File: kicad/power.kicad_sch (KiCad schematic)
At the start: 79 parts, among them J3 Conn_01x01_Pin, J9 Conn_01x02_Pin, U11 AMS1117-5.0, U12 ACS711xEXLT-15AB, U13 LM2937xMP, U15 MAX40200AUK, U7 AMS1117-3.3, U8 ACS711xEXLT-15AB, U9 ACS711xEXLT-15AB

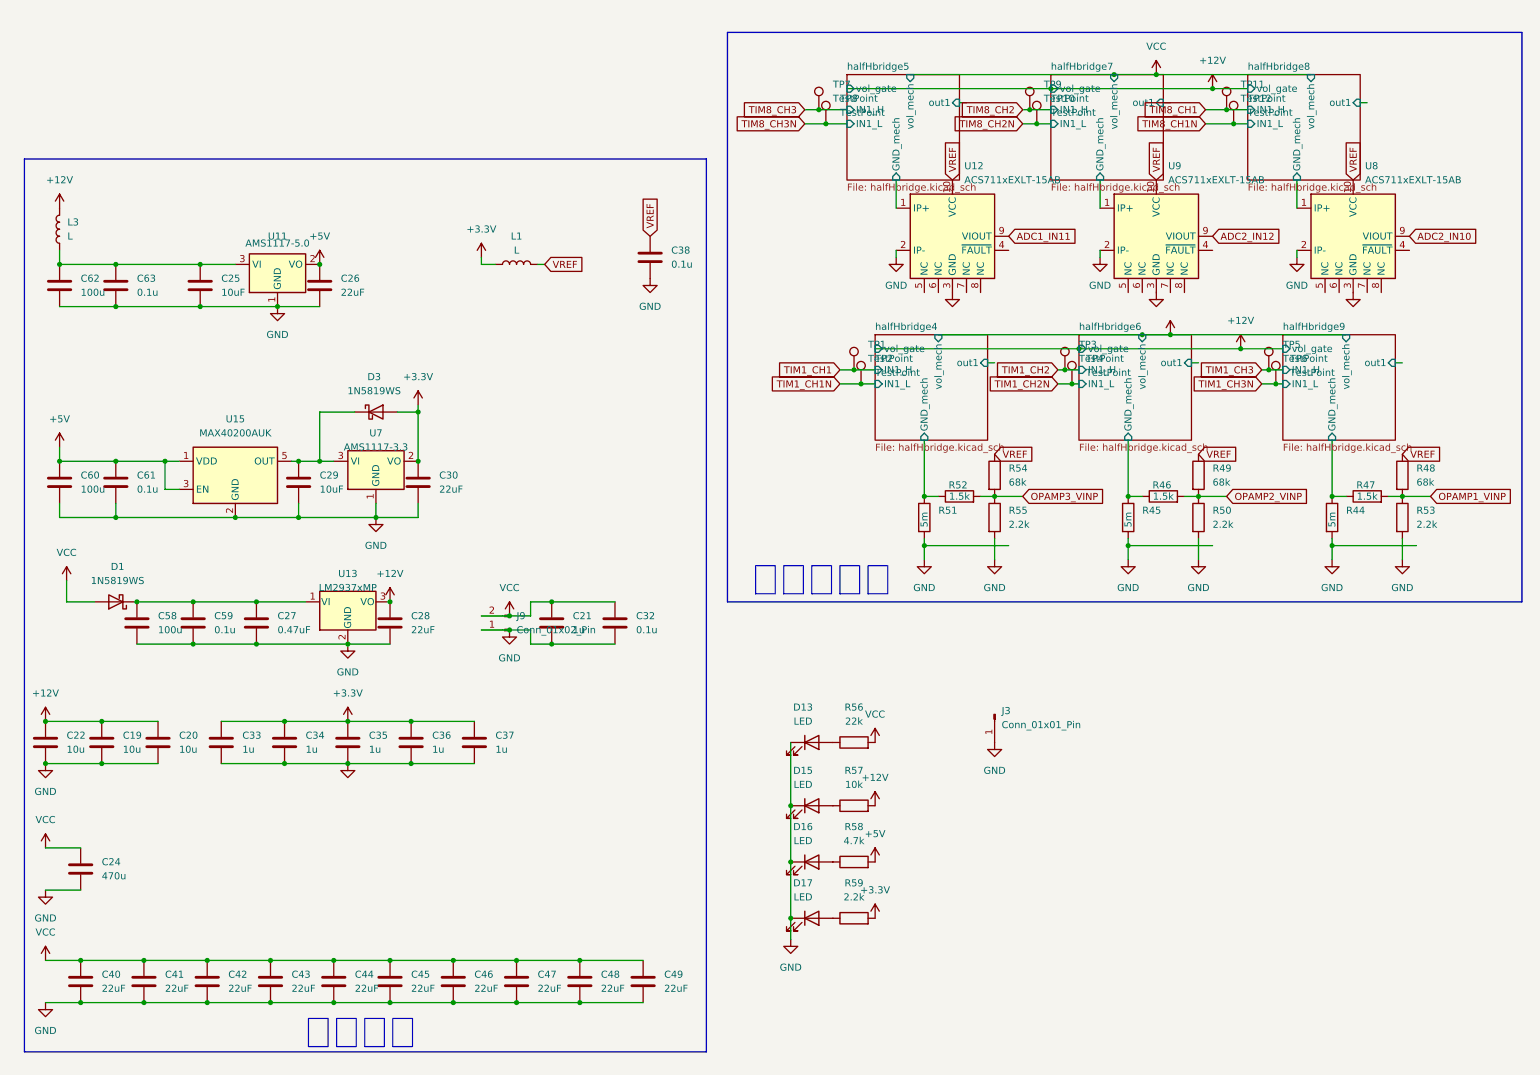
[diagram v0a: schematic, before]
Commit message: a
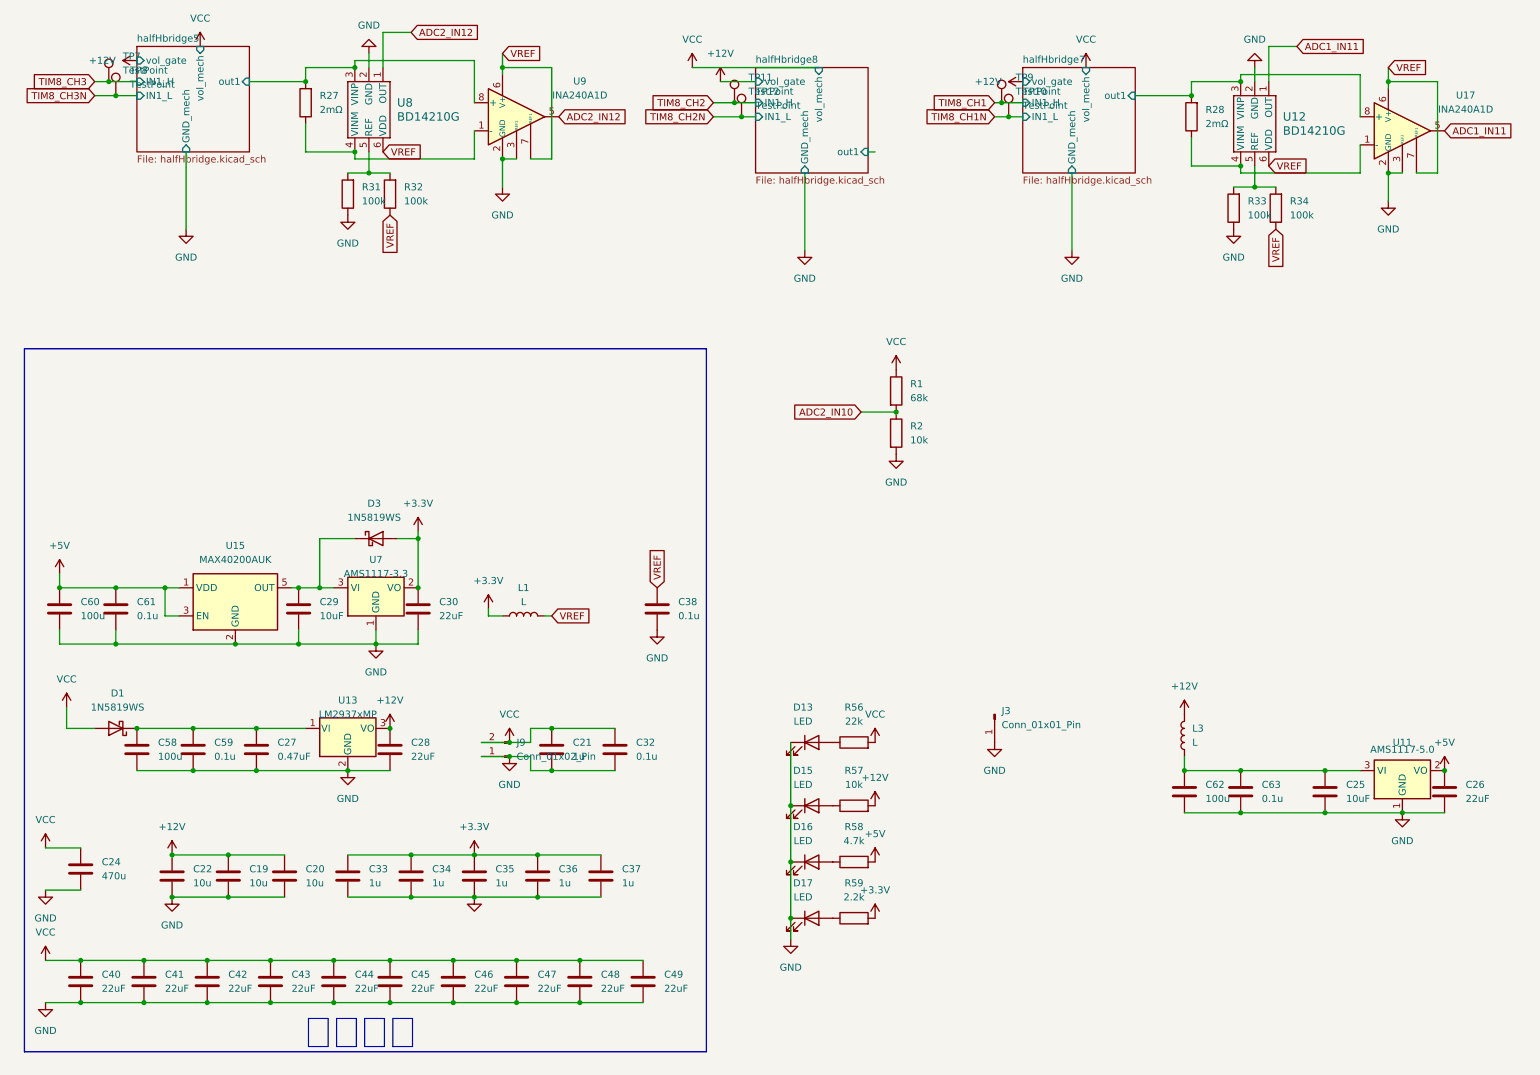
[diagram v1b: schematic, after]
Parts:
- removed R44, R45, R51: 5m, Resistor_SMD:R_2010_5025Metric_Pad1.40x2.65mm_HandSolder, symbol Device:R
- removed R46, R47, R52: 1.5k, Resistor_SMD:R_0402_1005Metric_Pad0.72x0.64mm_HandSolder, symbol Device:R
- removed R48, R49, R54: 68k, Resistor_SMD:R_0402_1005Metric_Pad0.72x0.64mm_HandSolder, symbol Device:R
- removed R50, R53, R55: 2.2k, Resistor_SMD:R_0402_1005Metric_Pad0.72x0.64mm_HandSolder, symbol Device:R
- removed TP1, TP2, TP3, TP4, TP5, TP6: TestPoint, TestPoint:TestPoint_Pad_D1.0mm, symbol Connector:TestPoint
- removed U12, U8, U9: ACS711xEXLT-15AB, Sensor_Current:Allegro_QFN-12-10-1EP_3x3mm_P0.5mm, symbol Sensor_Current:ACS711xEXLT-15AB
- added R1: 68k, Resistor_SMD:R_0402_1005Metric_Pad0.72x0.64mm_HandSolder, symbol Device:R
- added R2: 10k, Resistor_SMD:R_0402_1005Metric_Pad0.72x0.64mm_HandSolder, symbol Device:R
- added R27, R28: 2mΩ, Resistor_SMD:R_2010_5025Metric_Pad1.40x2.65mm_HandSolder, symbol Device:R
- added R31, R32, R33, R34: 100k, Resistor_SMD:R_0402_1005Metric_Pad0.72x0.64mm_HandSolder, symbol Device:R
- added U12, U8: BD14210G, footprints:SSOP6, symbol jisaku:BD14210G
- added U17, U9: INA240A1D, Package_SO:SOIC-8_3.9x4.9mm_P1.27mm, symbol Amplifier_Current:INA240A1D
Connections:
- net ADC1_IN11: now also U12.1 (OUT), U17.5
- net ADC2_IN10: now also R1.2, R2.1
- net ADC2_IN12: now also U8.1 (OUT), U9.5
- net GND: now also R2.2, R31.1, R33.1, U12.2 (GND), U17.2 (GND), U17.3 (REF2), U17.4 (GND), U8.2 (GND), U9.2 (GND), U9.3 (REF2), U9.4 (GND)
- net TIM8_CH1: now also TP9.1; no longer TP11.1
- net TIM8_CH1N: now also TP10.1; no longer TP12.1
- net TIM8_CH2: now also TP11.1; no longer TP9.1
- net TIM8_CH2N: now also TP12.1; no longer TP10.1
- net VCC: now also R1.1
- net VREF: now also R32.1, R34.1, U12.6 (VDD), U17.6 (V+), U17.7 (REF1), U8.6 (VDD), U9.6 (V+), U9.7 (REF1)
- net halfHbridge5/out1: now also R27.2, U8.3 (VINP), U9.8 (+)
- net halfHbridge7/out1: now also R28.2, U12.3 (VINP), U17.8 (+)
- new net: R33.2, R34.2, U12.5 (REF)
- new net: R27.1, U8.4 (VINM), U9.1 (-)
- new net: R31.2, R32.2, U8.5 (REF)
- new net: R28.1, U12.4 (VINM), U17.1 (-)
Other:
- removed sheet halfHbridge4
- removed sheet halfHbridge6
- removed sheet halfHbridge9
- note removed: "パワー回路"
- moved on the sheet: C19, C20, C21, C22, C25, C26, C27, C28, C29, C30, C32, C33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
